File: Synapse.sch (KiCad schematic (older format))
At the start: 7 parts, among them U1 WeAct_BlackPill

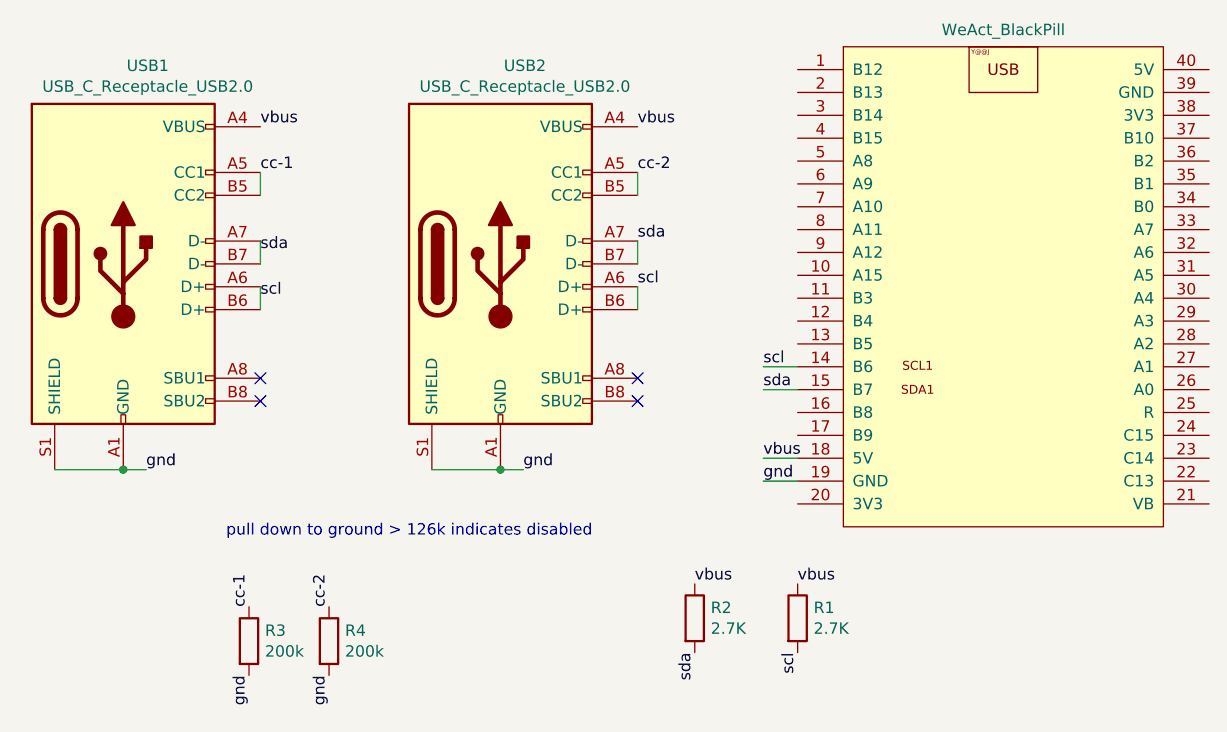
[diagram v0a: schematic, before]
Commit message: synapse mini
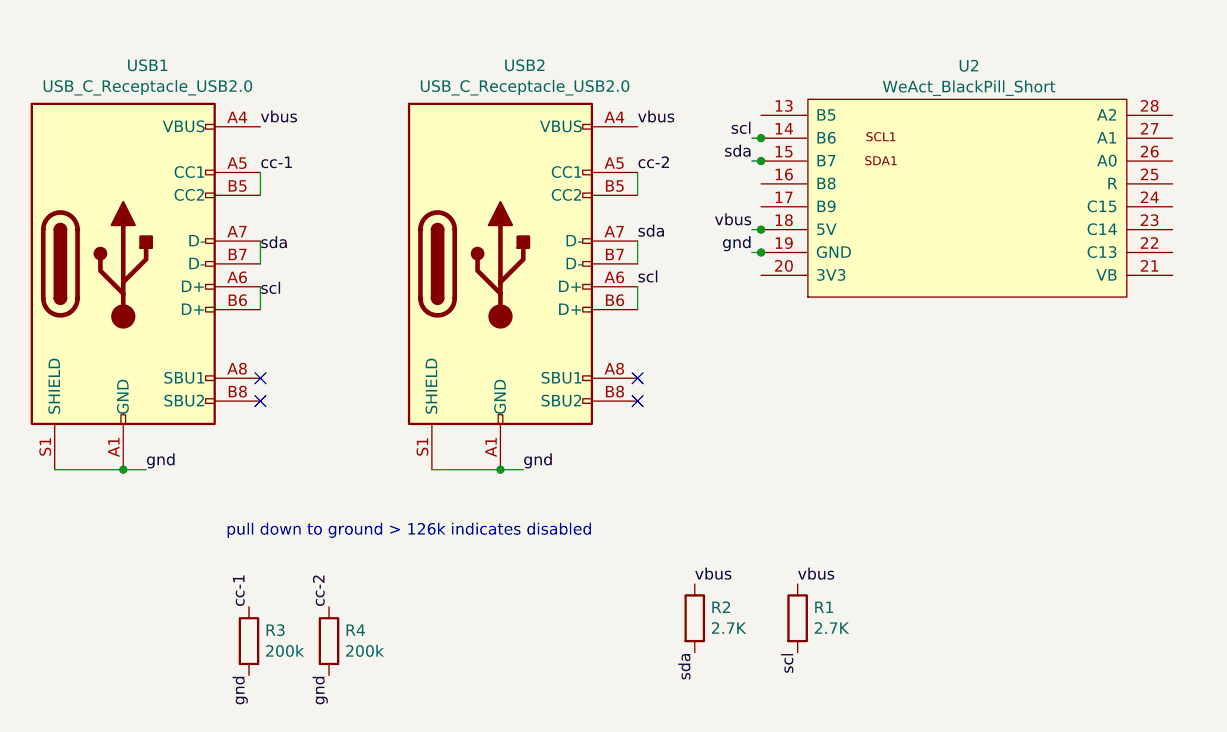
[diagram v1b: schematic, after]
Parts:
- removed U1: WeAct_BlackPill, Footprints:YAAJ_BluePill_2, symbol YAAJ_BlackPill:WeAct_BlackPill
- added U2: WeAct_BlackPill_Short, Footprints:BlackPill_Short, symbol YAAJ_BlackPill:WeAct_BlackPill_Short
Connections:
- wire segments 14 -> 18
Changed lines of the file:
@@
 	1    0    0    -1
 $EndComp
-Wire Wire Line
-	5950 3150 5800 3150
 $Comp
 L Connector:USB_C_Receptacle_USB2.0 USB1
@@
 Wire Wire Line
 	2700 3100 3000 3100
-Text Label 5800 3150 0    50   ~ 0
+Text Label 5750 2150 2    50   ~ 0
 gnd
-Text Label 5800 3050 0    50   ~ 0
+Text Label 5750 2050 2    50   ~ 0
 vbus
 Text Label 5250 2100 0    50   ~ 0
 sda
-Text Label 5800 2750 0    50   ~ 0
+Text Label 5750 1750 2    50   ~ 0
 sda
 Text Label 5250 1600 0    50   ~ 0
@@
 Text Label 5950 3900 3    50   ~ 0
 scl
-Text Label 5800 2650 0    50   ~ 0
+Text Label 5750 1650 2    50   ~ 0
 scl
-Wire Wire Line
-	5800 2650 5950 2650
-Wire Wire Line
-	5800 3050 5950 3050
 Text Label 4750 3100 0    50   ~ 0
 gnd
@@
 Wire Wire Line
 	3600 2100 3600 2200
-Wire Wire Line
-	5950 2750 5800 2750
 Text Label 3600 2350 0    50   ~ 0
 scl
@@
 Wire Wire Line
 	5250 2400 5250 2300
-$Comp
-L YAAJ_BlackPill:WeAct_BlackPill U1
-U 1 1 60EFFF91
-P 6850 2250
-F 0 "U1" H 6850 3415 50  0001 C CNN
-F 1 "WeAct_BlackPill" H 6850 3324 50  0000 C CNN
-F 2 "Footprints:YAAJ_BluePill_2" H 7650 1250 50  0001 C CNN
-F 3 "" H 7650 1250 50  0001 C CNN
-	1    6850 2250
-	1    0    0    -1
-$EndComp
 NoConn ~ 5250 2700
 NoConn ~ 5250 2800
@@
 Text Label 3900 4000 3    50   ~ 0
 gnd
+$Comp
+L YAAJ_BlackPill:WeAct_BlackPill_Short U2
+U 1 1 60F02FCD
+P 6700 1950
+F 0 "U2" H 6700 2565 50  0000 C CNN
+F 1 "WeAct_BlackPill_Short" H 6700 2474 50  0000 C CNN
+F 2 "Footprints:BlackPill_Short" H 7500 1630 50  0001 C CNN
+F 3 "" H 7500 1630 50  0001 C CNN
+	1    6700 1950
+	1    0    0    -1
+$EndComp
+Wire Wire Line
+	5800 1650 5790 1650
+Connection ~ 5790 1650
+Wire Wire Line
+	5790 1650 5750 1650
+Wire Wire Line
+	5800 1750 5790 1750
+Connection ~ 5790 1750
+Wire Wire Line
+	5790 1750 5750 1750
+Wire Wire Line
+	5800 2050 5790 2050
+Connection ~ 5790 2050
+Wire Wire Line
+	5790 2050 5750 2050
+Wire Wire Line
+	5800 2150 5790 2150
+Connection ~ 5790 2150
+Wire Wire Line
+	5790 2150 5750 2150
 $EndSCHEMATC
